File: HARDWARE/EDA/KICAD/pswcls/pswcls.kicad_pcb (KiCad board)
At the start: 2 copper layers, 26.5 x 29.9 mm, 13 parts, among them J1 CONN, J3 RELAY_TERMINAL, K1 SRA-12VDC-CL-REMIX, Q1 BC549, U1 4N35

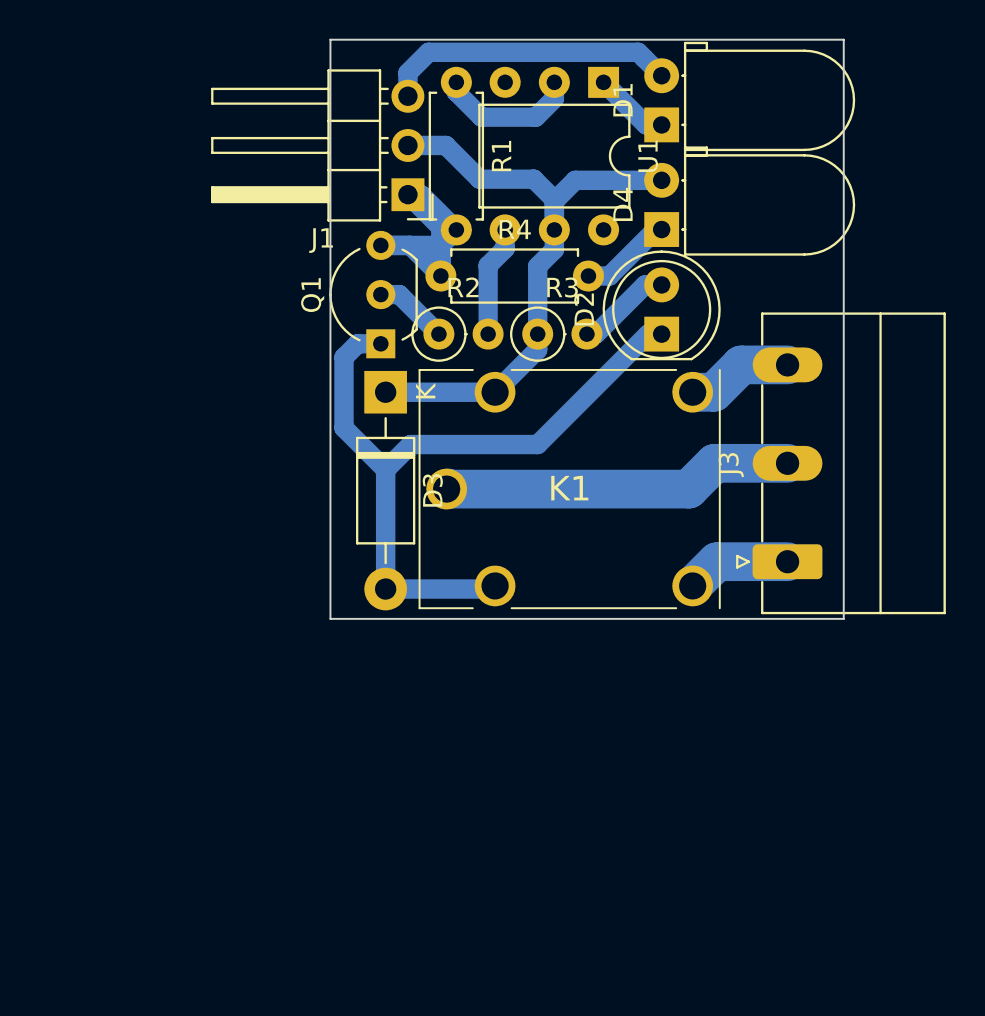
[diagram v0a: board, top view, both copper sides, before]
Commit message: adjust
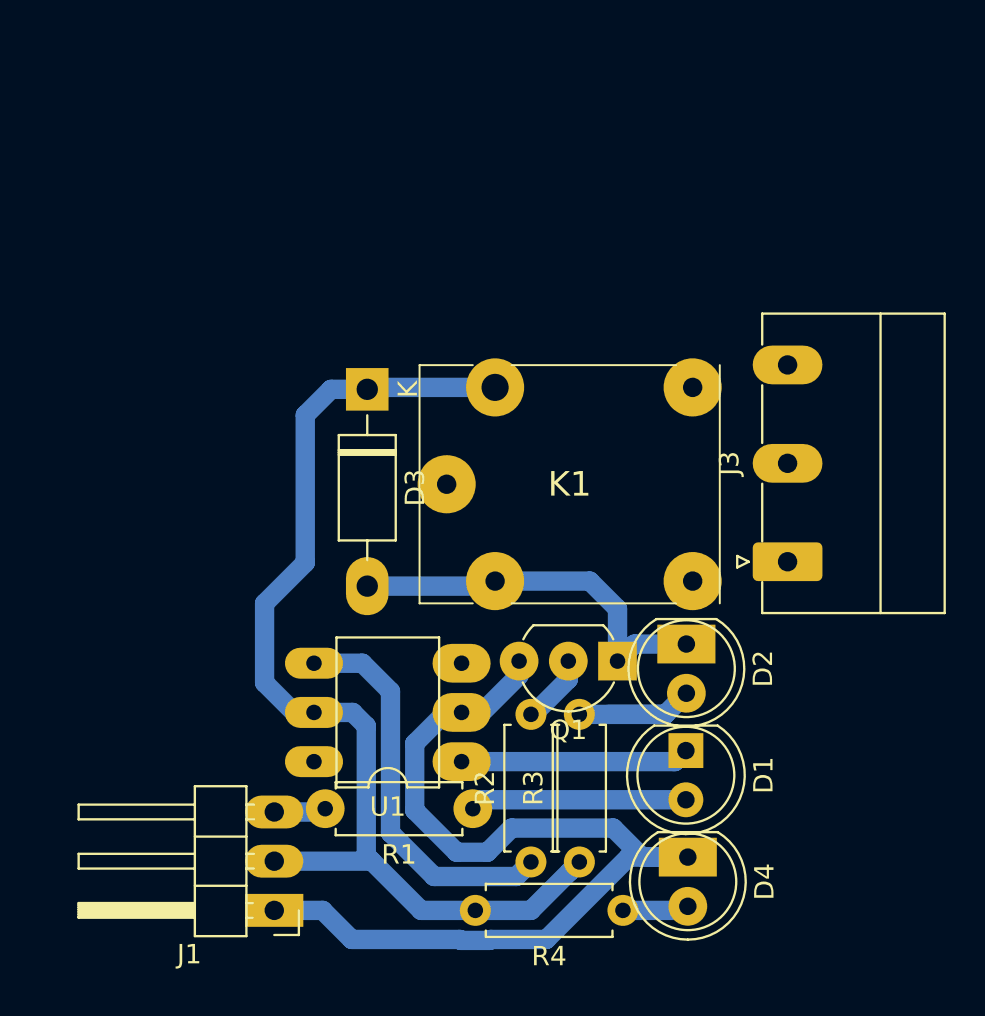
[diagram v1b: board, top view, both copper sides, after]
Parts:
- D1: footprint LED_THT:LED_D5.0mm_Horizontal_O1.27mm_Z3.0mm_Clear -> LED_THT:LED_D5.0mm_FlatTop
- D4: footprint LED_THT:LED_D5.0mm_Horizontal_O1.27mm_Z3.0mm -> LED_THT:LED_D5.0mm_Clear
- R2, R3: footprint Resistor_THT:R_Axial_DIN0207_L6.3mm_D2.5mm_P2.54mm_Vertical -> Resistor_THT:R_Axial_DIN0207_L6.3mm_D2.5mm_P7.62mm_Horizontal
- moved J1 37.6 mm to (143.5, 127.2)
- moved R1 37.5 mm to (153.8, 122.0), turned to 180 degrees
- moved U1 35.8 mm to (153.2, 119.6), turned to 180 degrees
- moved R4 34.1 mm to (161.5, 127.2), turned to 180 degrees
- moved D4 32.4 mm to (164.8, 124.5), turned to 270 degrees
- moved D1 32.3 mm to (164.8, 119.0), turned to 270 degrees
- moved R2 27.7 mm to (156.8, 124.8), turned to 90 degrees
- moved R3 27.3 mm to (159.2, 124.8), turned to 90 degrees
- moved Q1 20.4 mm to (161.2, 114.4), turned to 180 degrees
- moved D2 16.1 mm to (164.8, 113.5), turned to 270 degrees
- moved D3 0.96 mm to (148.3, 100.3)
- moved K1 0.25 mm to (158.8, 105.2)
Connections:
- D1 pad 2: vll_relay -> Net-(D1-Pad2)
- D4 pad 1: Net-(D4-Pad1) -> GNDA
- D4 pad 2: vcc_relay -> Net-(D4-Pad2)
- R1 pad 1: Net-(R1-Pad1) -> Net-(D1-Pad2)
- R1 pad 2: GNDA -> vll_relay
- R2 pad 1: Net-(Q1-Pad2) -> Net-(R2-Pad1)
- R2 pad 2: Net-(R2-Pad2) -> Net-(Q1-Pad2)
- R4 pad 1: GNDA -> Net-(D4-Pad2)
- R4 pad 2: Net-(D4-Pad1) -> vcc_relay
- U1 pad 2: Net-(R1-Pad1) -> GNDA
- U1 pad 4: Net-(R2-Pad2) -> Net-(R2-Pad1)
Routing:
- net GNDA: track 17.7 -> 50.9 mm
- net vcc_relay: track 33.9 -> 56.2 mm
- net Net-(R2-Pad1): track 0.00 -> 20.4 mm
- net C_Relay: track 18.2 -> 0.00 mm
- net Net-(D2-Pad1): track 37.9 -> 20.2 mm
- net vll_relay: track 15.2 -> 2.80 mm
- net Net-(D1-Pad2): track 0.00 -> 11.2 mm
- net Net-(D1-Pad1): track 3.91 -> 11.8 mm
- net Net-(R1-Pad1): track 7.34 -> 0.00 mm
- net Net-(R2-Pad2): track 5.74 -> 0.00 mm
- net NA_Relay: track 5.48 -> 0.00 mm
- net NC_Relay: track 5.42 -> 0.00 mm
- net Net-(D4-Pad1): track 5.27 -> 0.00 mm
- net Net-(D2-Pad2): track 4.91 -> 8.91 mm
- net Net-(D4-Pad2): track 0.00 -> 3.44 mm
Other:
- board outline removed

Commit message: pause
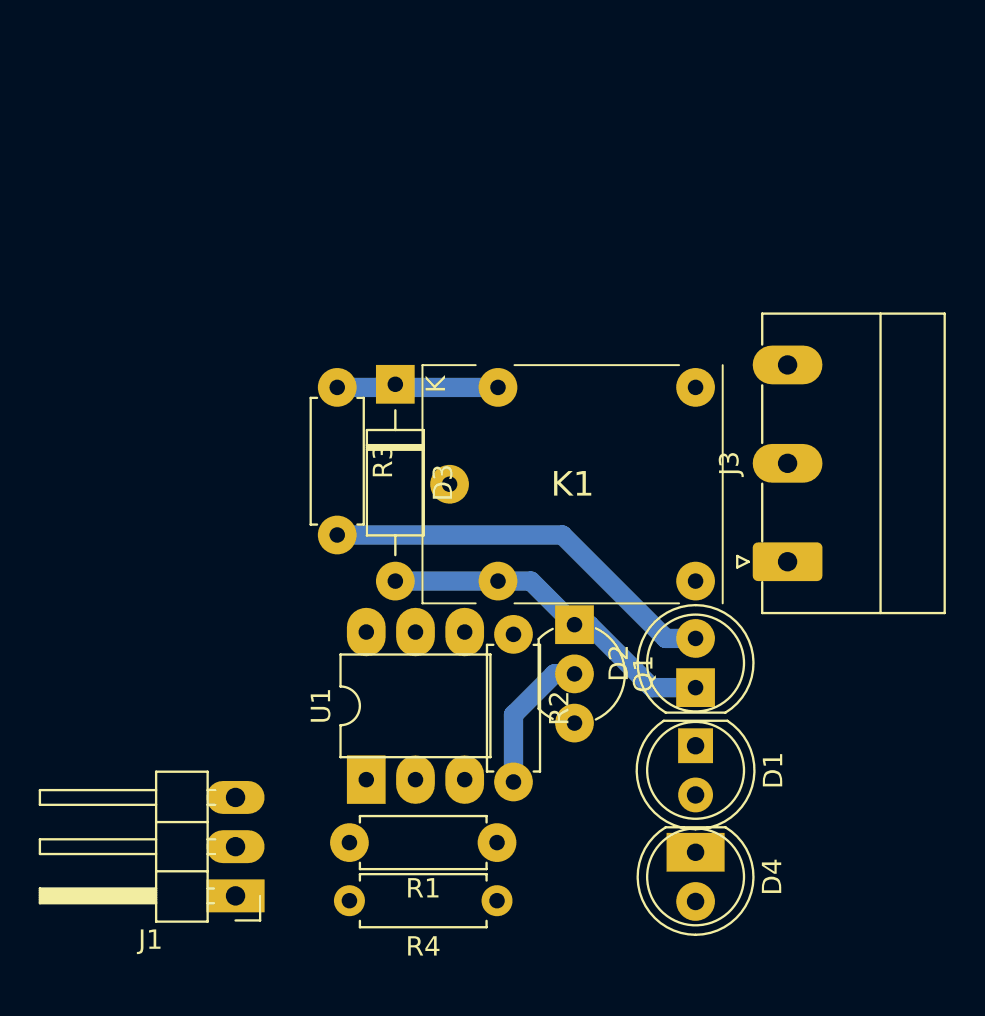
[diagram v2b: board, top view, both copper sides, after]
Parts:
- moved R3 27.5 mm to (146.8, 100.2), turned to 270 degrees
- moved R2 11.8 mm to (155.8, 113.0), turned to 270 degrees
- moved R4 6.52 mm to (155.0, 126.8)
- moved U1 5.01 mm to (148.2, 120.5), turned to 90 degrees
- moved Q1 2.91 mm to (159.0, 112.5), turned to 270 degrees
- moved D2 2.30 mm to (165.2, 115.8), turned to 90 degrees
- moved R1 2.15 mm to (155.0, 123.8)
- moved J1 2.14 mm to (141.5, 126.5)
- moved D3 1.47 mm to (149.8, 100.1)
- moved D1 0.56 mm to (165.2, 118.8)
- moved D4 0.47 mm to (165.2, 124.2)
- moved K1 0.15 mm to (158.9, 105.2)
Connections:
- U1 pad 3: (no net) -> Net-(U1-Pad3)
- U1 pad 6: (no net) -> Net-(U1-Pad6)
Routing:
- net GNDA: track 50.9 -> 0.00 mm
- net vcc_relay: track 56.2 -> 8.43 mm
- net Net-(R2-Pad1): track 20.4 -> 0.00 mm
- net Net-(D1-Pad1): track 11.8 -> 0.00 mm
- net Net-(D2-Pad2): track 8.91 -> 20.7 mm
- net Net-(D1-Pad2): track 11.2 -> 0.00 mm
- net Net-(Q1-Pad2): track 3.62 -> 7.49 mm
- net Net-(D4-Pad2): track 3.44 -> 0.00 mm
- net vll_relay: track 2.80 -> 0.00 mm
- net Net-(D2-Pad1): track 20.2 -> 17.8 mm

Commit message: adjust complete
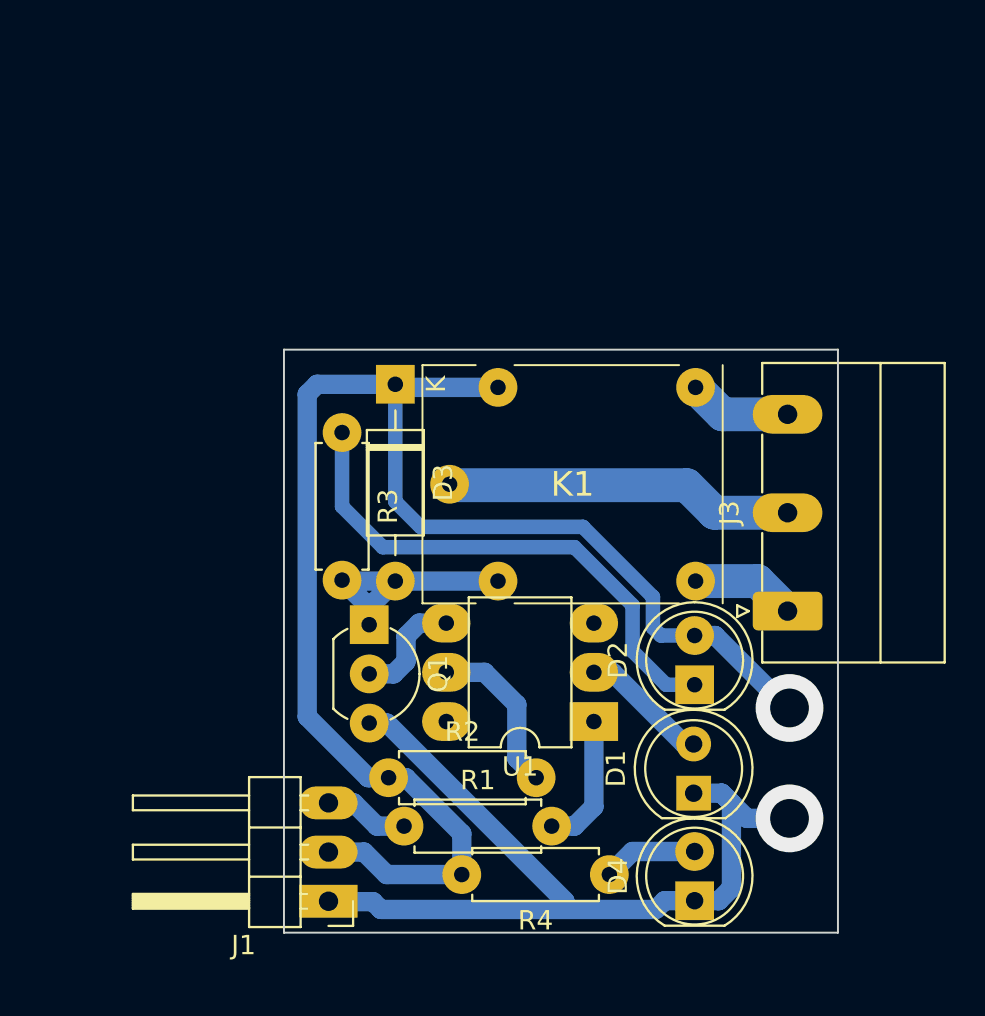
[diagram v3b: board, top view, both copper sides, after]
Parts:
- moved U1 12.1 mm to (160.0, 117.5), turned to 180 degrees
- moved Q1 10.6 mm to (148.4, 112.5)
- moved R2 9.82 mm to (149.4, 120.4), turned to 0 degrees
- moved R4 5.96 mm to (160.8, 125.4)
- moved R1 4.87 mm to (150.2, 122.9), turned to 0 degrees
- moved J1 4.81 mm to (146.3, 126.8)
- moved J3 2.55 mm to (170.0, 111.8)
- moved D4 2.50 mm to (165.2, 126.8), turned to 90 degrees
- moved D1 2.45 mm to (165.2, 121.2), turned to 90 degrees
- moved R3 2.34 mm to (147.0, 102.6)
- moved D2 0.16 mm to (165.2, 115.6)
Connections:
- D1 pad 1: Net-(D1-Pad1) -> GNDA
- D2 pad 2: Net-(D2-Pad2) -> vcc_relay
- D3 pad 2: Net-(D2-Pad1) -> Net-(D3-Pad2)
- K1 pad 5: Net-(D2-Pad1) -> Net-(D3-Pad2)
- Q1 pad 1: Net-(D2-Pad1) -> Net-(D3-Pad2)
- R1 pad 1: Net-(D1-Pad2) -> vll_relay
- R1 pad 2: vll_relay -> Net-(R1-Pad2)
- R2 pad 1: Net-(R2-Pad1) -> vcc_relay
- R2 pad 2: Net-(Q1-Pad2) -> Net-(R2-Pad2)
- R3 pad 1: vcc_relay -> Net-(D2-Pad1)
- R3 pad 2: Net-(D2-Pad2) -> Net-(D3-Pad2)
- U1 pad 1: Net-(D1-Pad1) -> Net-(R1-Pad2)
- U1 pad 2: GNDA -> Net-(D1-Pad2)
- U1 pad 3: Net-(U1-Pad3) -> (no net)
- U1 pad 4: Net-(R2-Pad1) -> Net-(Q1-Pad2)
- U1 pad 5: vcc_relay -> Net-(R2-Pad2)
- U1 pad 6: Net-(U1-Pad6) -> (no net)
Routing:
- net vcc_relay: track 8.43 -> 78.7 mm, vias 0 -> 1
- net GNDA: track 0.00 -> 47.3 mm, vias 0 -> 1
- net Net-(D2-Pad2): track 20.7 -> 0.00 mm
- net C_Relay: track 0.00 -> 18.1 mm
- net Net-(D3-Pad2): track 0.00 -> 13.5 mm
- net Net-(D2-Pad1): track 17.8 -> 27.2 mm
- net Net-(R2-Pad2): track 0.00 -> 8.52 mm
- net Net-(R1-Pad2): track 0.00 -> 7.19 mm
- net Net-(D1-Pad2): track 0.00 -> 6.68 mm
- net NC_Relay: track 0.00 -> 5.39 mm
- net NA_Relay: track 0.00 -> 5.33 mm
- net Net-(D4-Pad2): track 0.00 -> 4.89 mm
- net vll_relay: track 0.00 -> 4.40 mm
- net Net-(Q1-Pad2): track 7.49 -> 5.83 mm
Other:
- board outline added: 28.6 x 30.1 mm
- net class Default: clearance 0.25 -> 0.3
- rule trace_clearance: 0.25 -> 0.3
